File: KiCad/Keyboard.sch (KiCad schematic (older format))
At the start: 77 parts, among them J1 USB_mini_micro_B, K1 KEYSW, K10 KEYSW, K11 KEYSW, K12 KEYSW, K13 KEYSW, K14 KEYSW, K15 KEYSW, K16 KEYSW, K17 KEYSW, K18 KEYSW, K19 KEYSW, K2 KEYSW, K20 KEYSW, K21 KEYSW, K22 KEYSW, K3 KEYSW, K4 KEYSW, K5 KEYSW, K6 KEYSW, K7 KEYSW, K8 KEYSW, K9 KEYSW, SW1 SW_PUSH, U1 ATMEGA32U4, X1 XTAL_GND

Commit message: Completed COl connectons an UG and KG LEDS started RE LED connections
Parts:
- removed D? (x13): WS2812, LED_SMD:LED_WS2812_PLCC6_5.0x5.0mm_P1.6mm, symbol LED:WS2812
- added KG1, KG10, KG11, KG12, KG13, KG14, KG15, KG16, KG17, KG18, KG19, KG2, KG20, KG21, KG22, KG3, KG4, KG5, KG6, KG7, KG8, KG9, UG1, UG10, UG11, UG12, UG13, UG14, UG2, UG3, UG4, UG5, UG6, UG7, UG8, UG9: WS2812B, LED_SMD:LED_WS2812B_PLCC4_5.0x5.0mm_P3.2mm, symbol LED:WS2812B
- added U? (x4): WS2811, symbol Driver_LED:WS2811
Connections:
- wire segments 186 -> 257
- no-connect marks 14 -> 13
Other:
- note added: "Key LEDs (KG1 - KG22)"
- note added: "Rotary Encoder LEDS (RE1 - RE4)"
- note added: "Underglow LEDs (UG1 - UG14)"

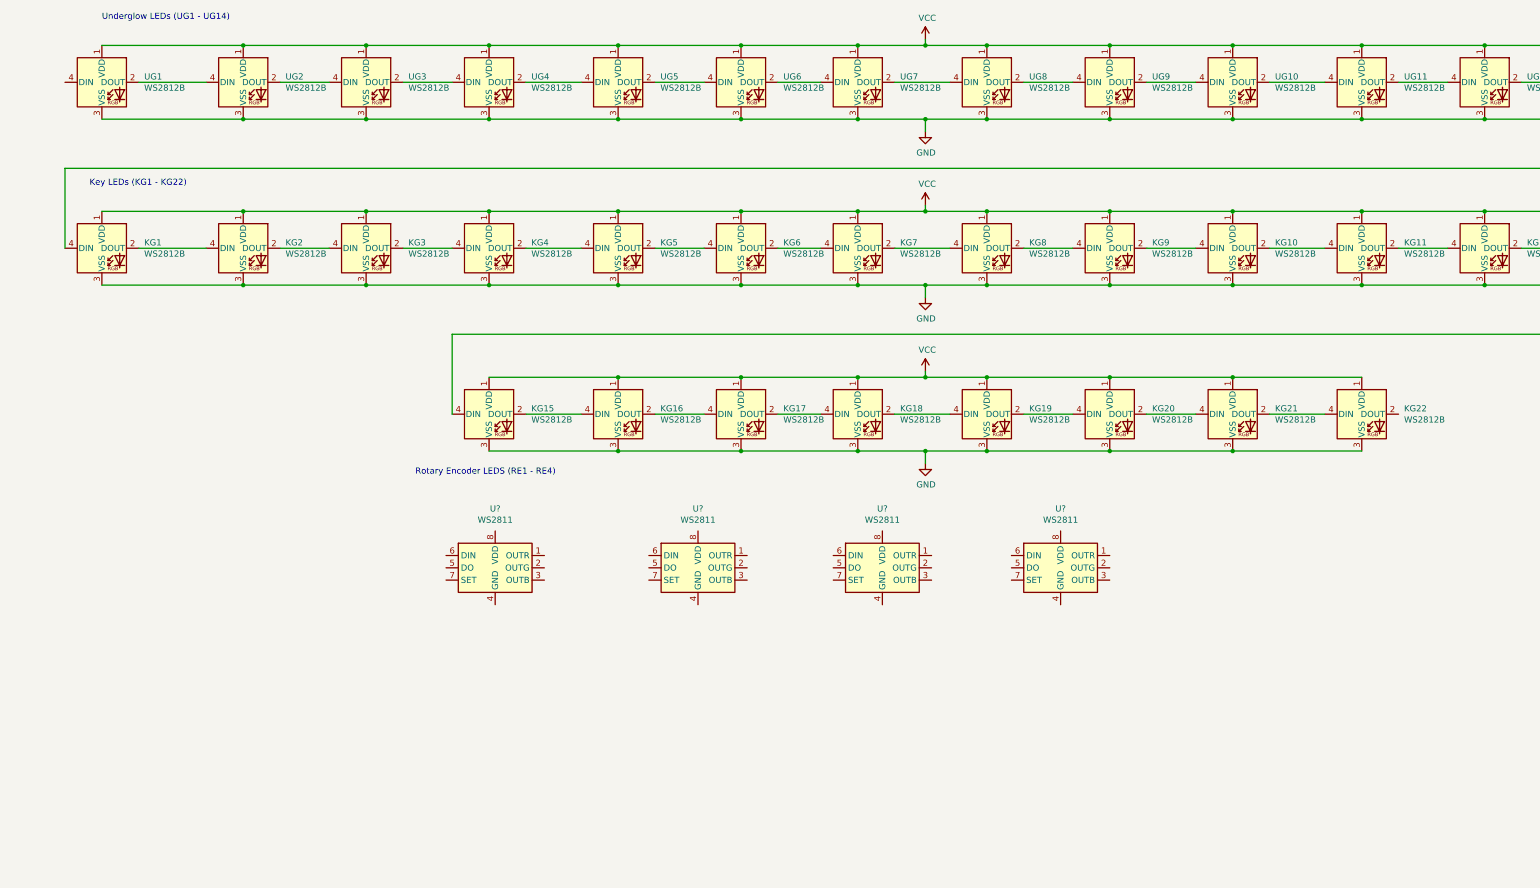
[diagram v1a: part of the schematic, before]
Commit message: A bit closer, ran out of pins on MCU ugh!!
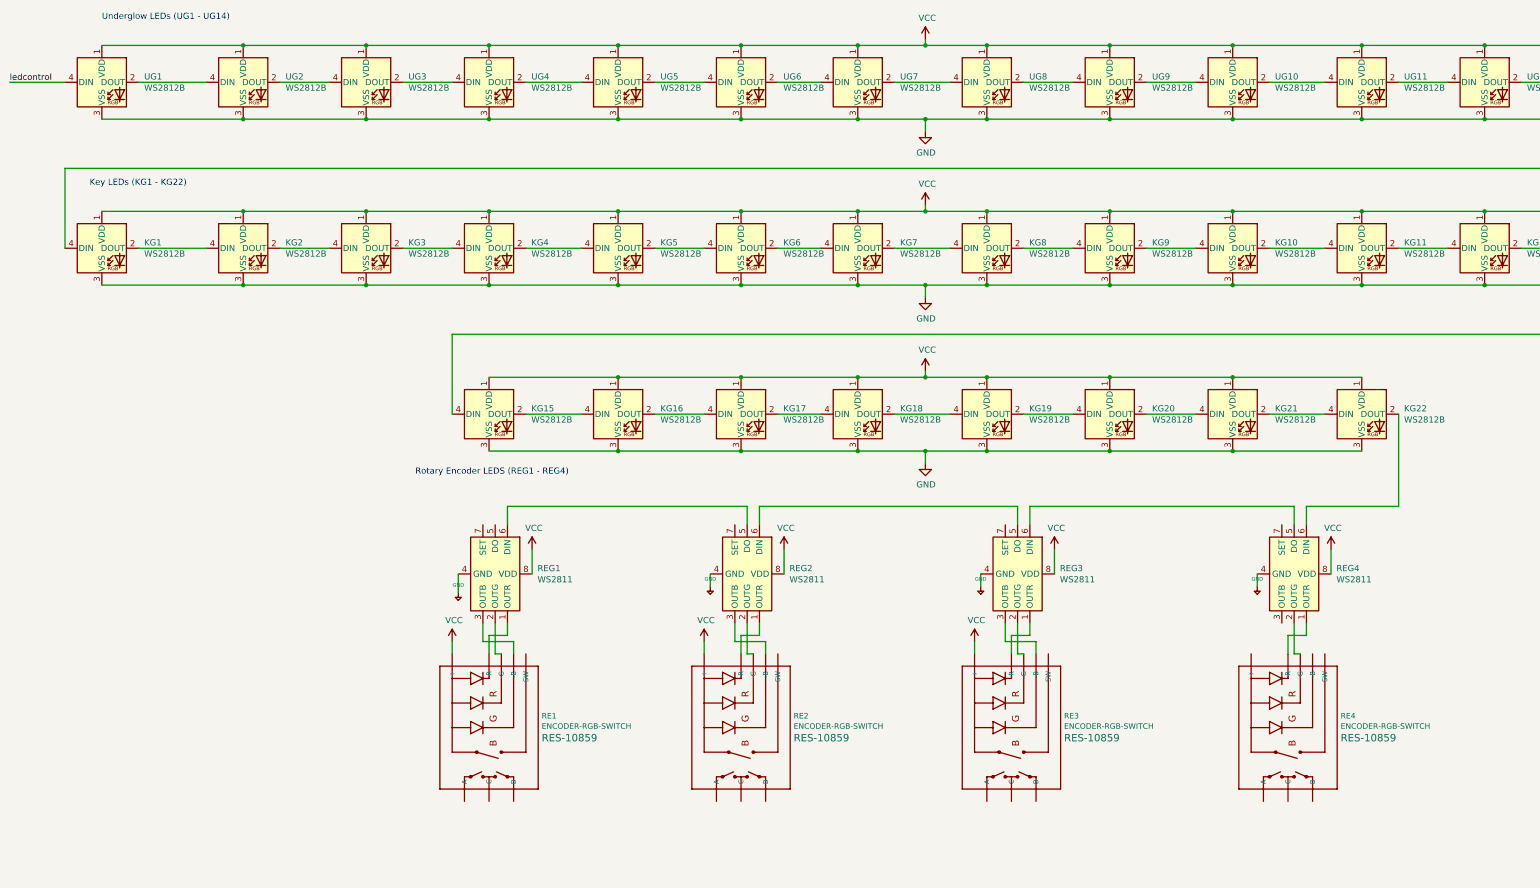
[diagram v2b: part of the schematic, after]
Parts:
- added RE1, RE2, RE3, RE4: ENCODER-RGB-SWITCH, ENCODER_LED_3, symbol SparkFun-Switches:ENCODER-RGB-SWITCH
- gave numbers to parts that had none: 4
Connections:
- net labels added: ledcontrol
- wire segments 257 -> 310
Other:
- note added: "Rotary Encoder LEDS (REG1 - REG4)"
- note removed: "Rotary Encoder LEDS (RE1 - RE4)"
- moved on the sheet: REG1, REG2, REG3, REG4

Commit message: all LEDs I think are setup, one question there in bold.
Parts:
- added C-KG1, C-KG10, C-KG11, C-KG12, C-KG13, C-KG14, C-KG15, C-KG16, C-KG17, C-KG18, C-KG19, C-KG2, C-KG20, C-KG21, C-KG22, C-KG3, C-KG4, C-KG5, C-KG6, C-KG7, C-KG8, C-KG9, C-REG1, C-REG2, C-REG3, C-REG4, C-UG1, C-UG10, C-UG11, C-UG12, C-UG13, C-UG14, C-UG2, C-UG3, C-UG4, C-UG5, C-UG6, C-UG7, C-UG8, C-UG9: 104, symbol Device:C
- added R-REG1, R-REG2, R-REG3, R-REG4: 100R, symbol Device:R
- added R-REG1, R-REG2, R-REG3, R-REG4: 33R, symbol Device:R
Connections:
- wire segments 310 -> 467
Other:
- note added: "R-REG4 is it needed"

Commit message: Changed to SMALL components
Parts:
- C-KG1, C-KG10, C-KG11, C-KG12, C-KG13, C-KG14, C-KG15, C-KG16, C-KG17, C-KG18, C-KG19, C-KG2, C-KG20, C-KG21, C-KG22, C-KG3, C-KG4, C-KG5, C-KG6, C-KG7, C-KG8, C-KG9, C-REG1, C-REG2, C-REG3, C-REG4, C-UG1, C-UG10, C-UG11, C-UG12, C-UG13, C-UG14, C-UG2, C-UG3, C-UG4, C-UG5, C-UG6, C-UG7, C-UG8, C-UG9: symbol Device:C -> Device:C_Small
- C10, C9: renamed from C?; symbol Device:C -> Device:C_Small
- C3, C4, C5, C6: value .1u -> 104
- D1, D10, D11, D12, D13, D14, D15, D16, D17, D18, D19, D2, D20, D21, D22, D3, D4, D5, D6, D7, D8, D9: symbol Device:D -> Device:D_Small
- R-REG1, R-REG2, R-REG3, R-REG4, R1, R2, R3, R4: symbol Device:R -> Device:R_Small
- R-VREG1: renamed from R-REG1; symbol Device:R -> Device:R_Small
- R-VREG2: renamed from R-REG2; symbol Device:R -> Device:R_Small
- R-VREG3: renamed from R-REG3; symbol Device:R -> Device:R_Small
- R-VREG4: renamed from R-REG4; symbol Device:R -> Device:R_Small
- gave numbers to parts that had none: 2
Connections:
- wire segments 467 -> 474
- no-connect marks 13 -> 18
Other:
- moved on the sheet: C3, C4, C5, C6, C7, J2, K1, K10, K11, K12, K13, K14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
